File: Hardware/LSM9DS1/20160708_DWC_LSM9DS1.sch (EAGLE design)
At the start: 8 parts, among them U1 LSM9DS1

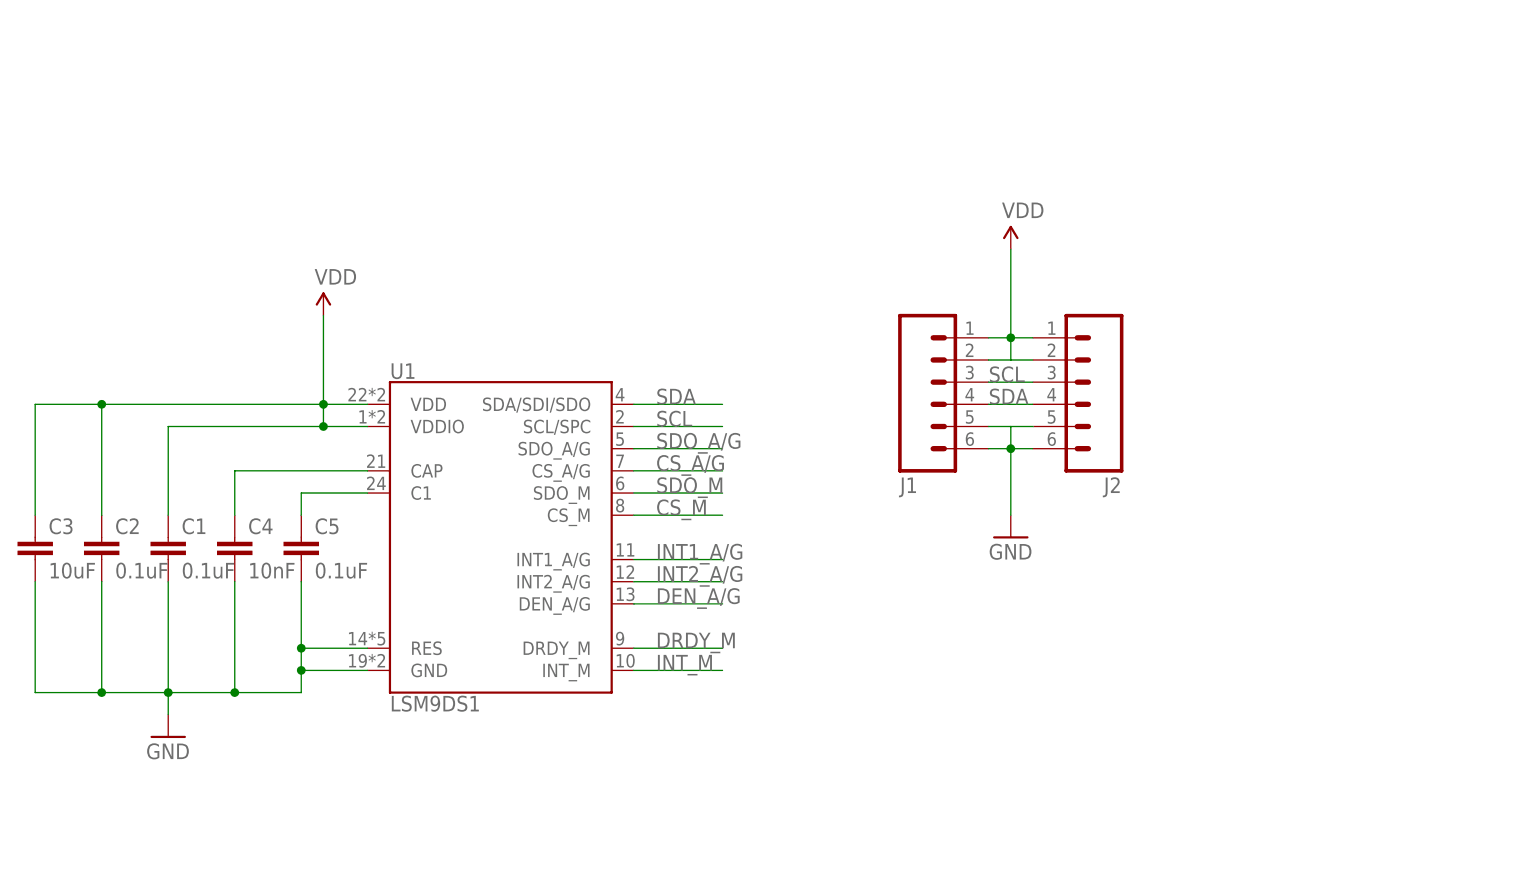
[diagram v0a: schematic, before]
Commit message: Rev 3 IMU Board
Here it is, in all its glory.
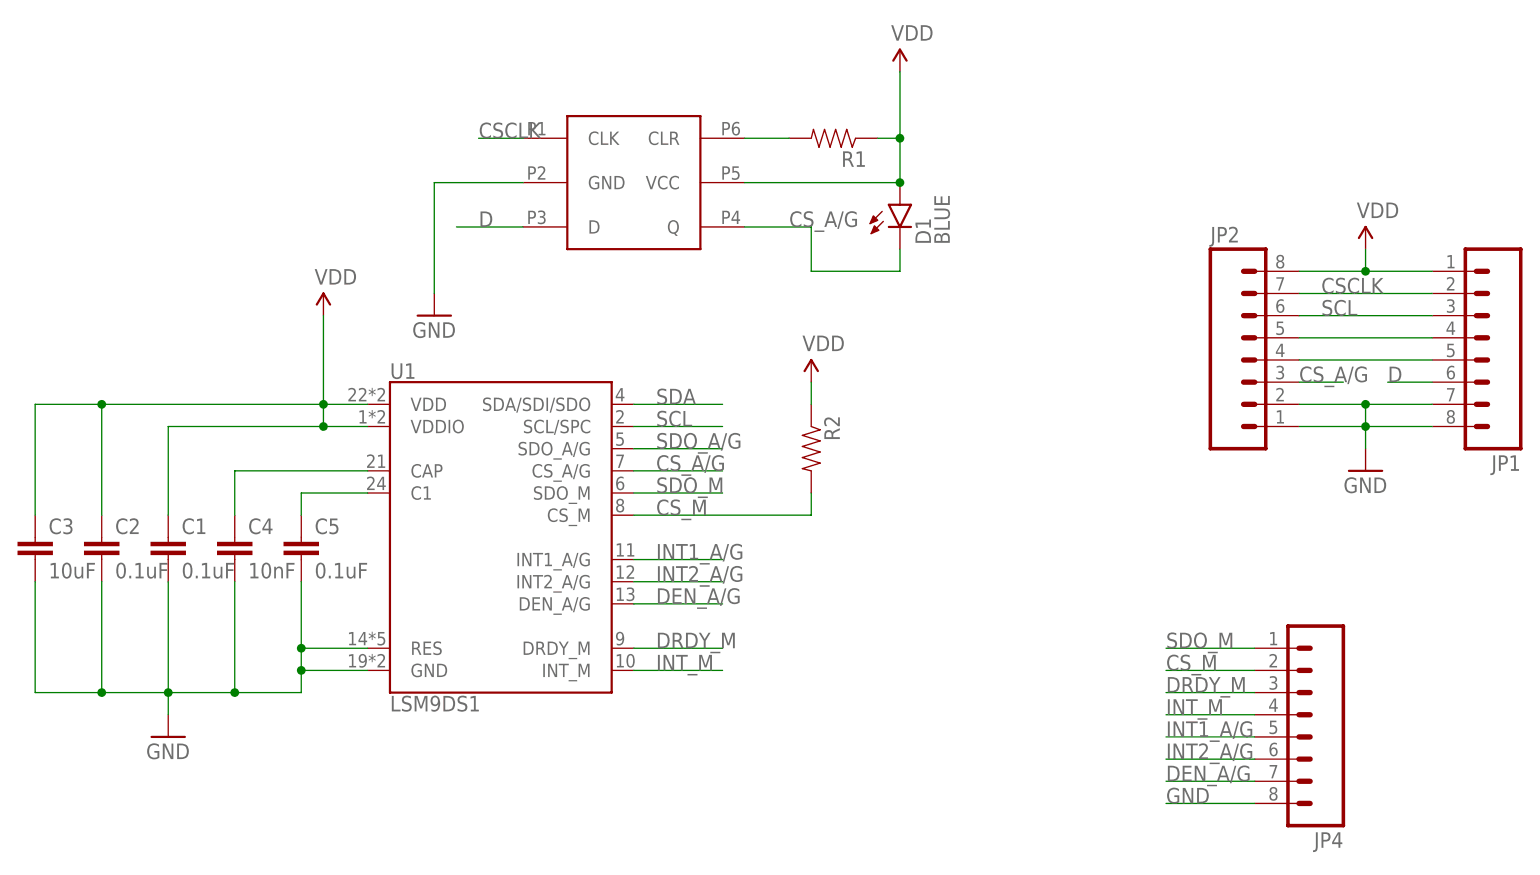
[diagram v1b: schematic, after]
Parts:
- removed J1, J2: (no value), SparkFun-Connectors:M06SMD-1MM
- added D1: BLUE, SparkFun-LED:LED-BLUE0603
- added JP1, JP2, JP4: (no value), SparkFun-Connectors:M08BM08B-SRSS-TB
- added R1, R2: (no value), SparkFun-Passives:RESISTOR0603-RES
- added U$1: SN74LVC1G175, CSL_Components:SN74LVC1G175
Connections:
- new net CSCLK: JP1.2, JP2.7, U$1.CLK
- new net D: JP1.6, U$1.D
- new net N$1: R1.2, U$1.CLR
- net CS_A/G: now also D1.C, JP2.3, U$1.Q
- net CS_M: now also JP4.2, R2.2
- net DEN_A/G: now also JP4.7
- net DRDY_M: now also JP4.3
- net GND: now also JP1.7, JP1.8, JP2.1, JP2.2, JP4.8, U$1.GND; no longer J1.5, J1.6, J2.5, J2.6
- net INT1_A/G: now also JP4.5
- net INT2_A/G: now also JP4.6
- net INT_M: now also JP4.4
- net SCL: now also JP1.3, JP2.6; no longer J1.3, J2.3
- net SDA: now also JP1.4, JP2.5; no longer J1.4, J2.4
- net SDO_A/G: now also JP1.5, JP2.4
- net SDO_M: now also JP4.1
- net VDD: now also D1.A, JP1.1, JP2.8, R1.1, R2.1, U$1.VCC; no longer J1.1, J1.2, J2.1, J2.2
